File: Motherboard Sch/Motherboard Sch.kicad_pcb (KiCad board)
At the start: 2 copper layers, 117.5 x 103.5 mm, 74 parts, among them J1 DIN-5, J2 Master ISCP, J3 E SLAVE ISCP, J4 E Slave Out, J6 Pluck ISCP, J7 Pick Unit, J8 Pluck Out, J9 Power In, SW2 Master Reset, SW3 E-slave Reset, SW4 Pluck Reset, U1 PIC16F1788, U2 PIC16F1789, U3 PIC16F1789, U4 LM1117MP-1.8

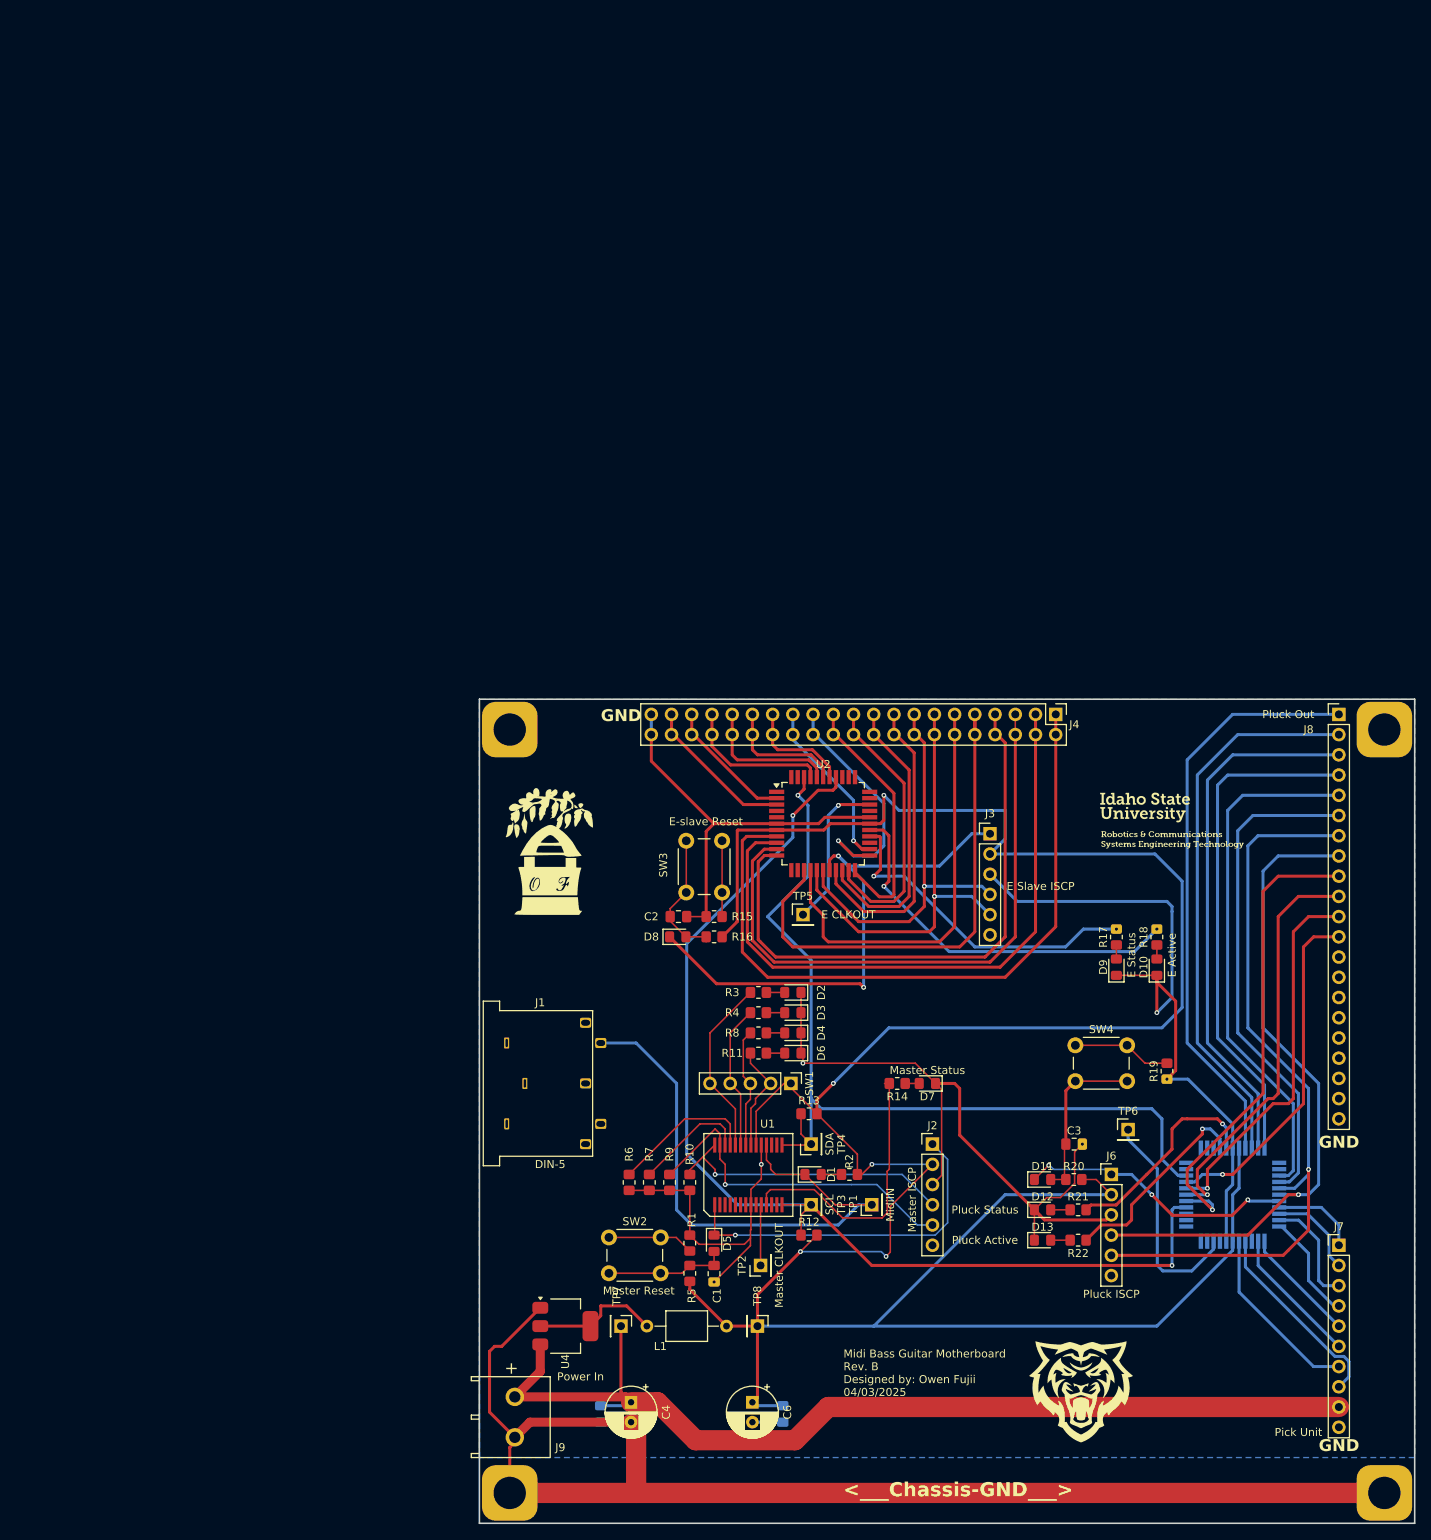
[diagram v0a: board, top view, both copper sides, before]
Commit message: added new report to repo
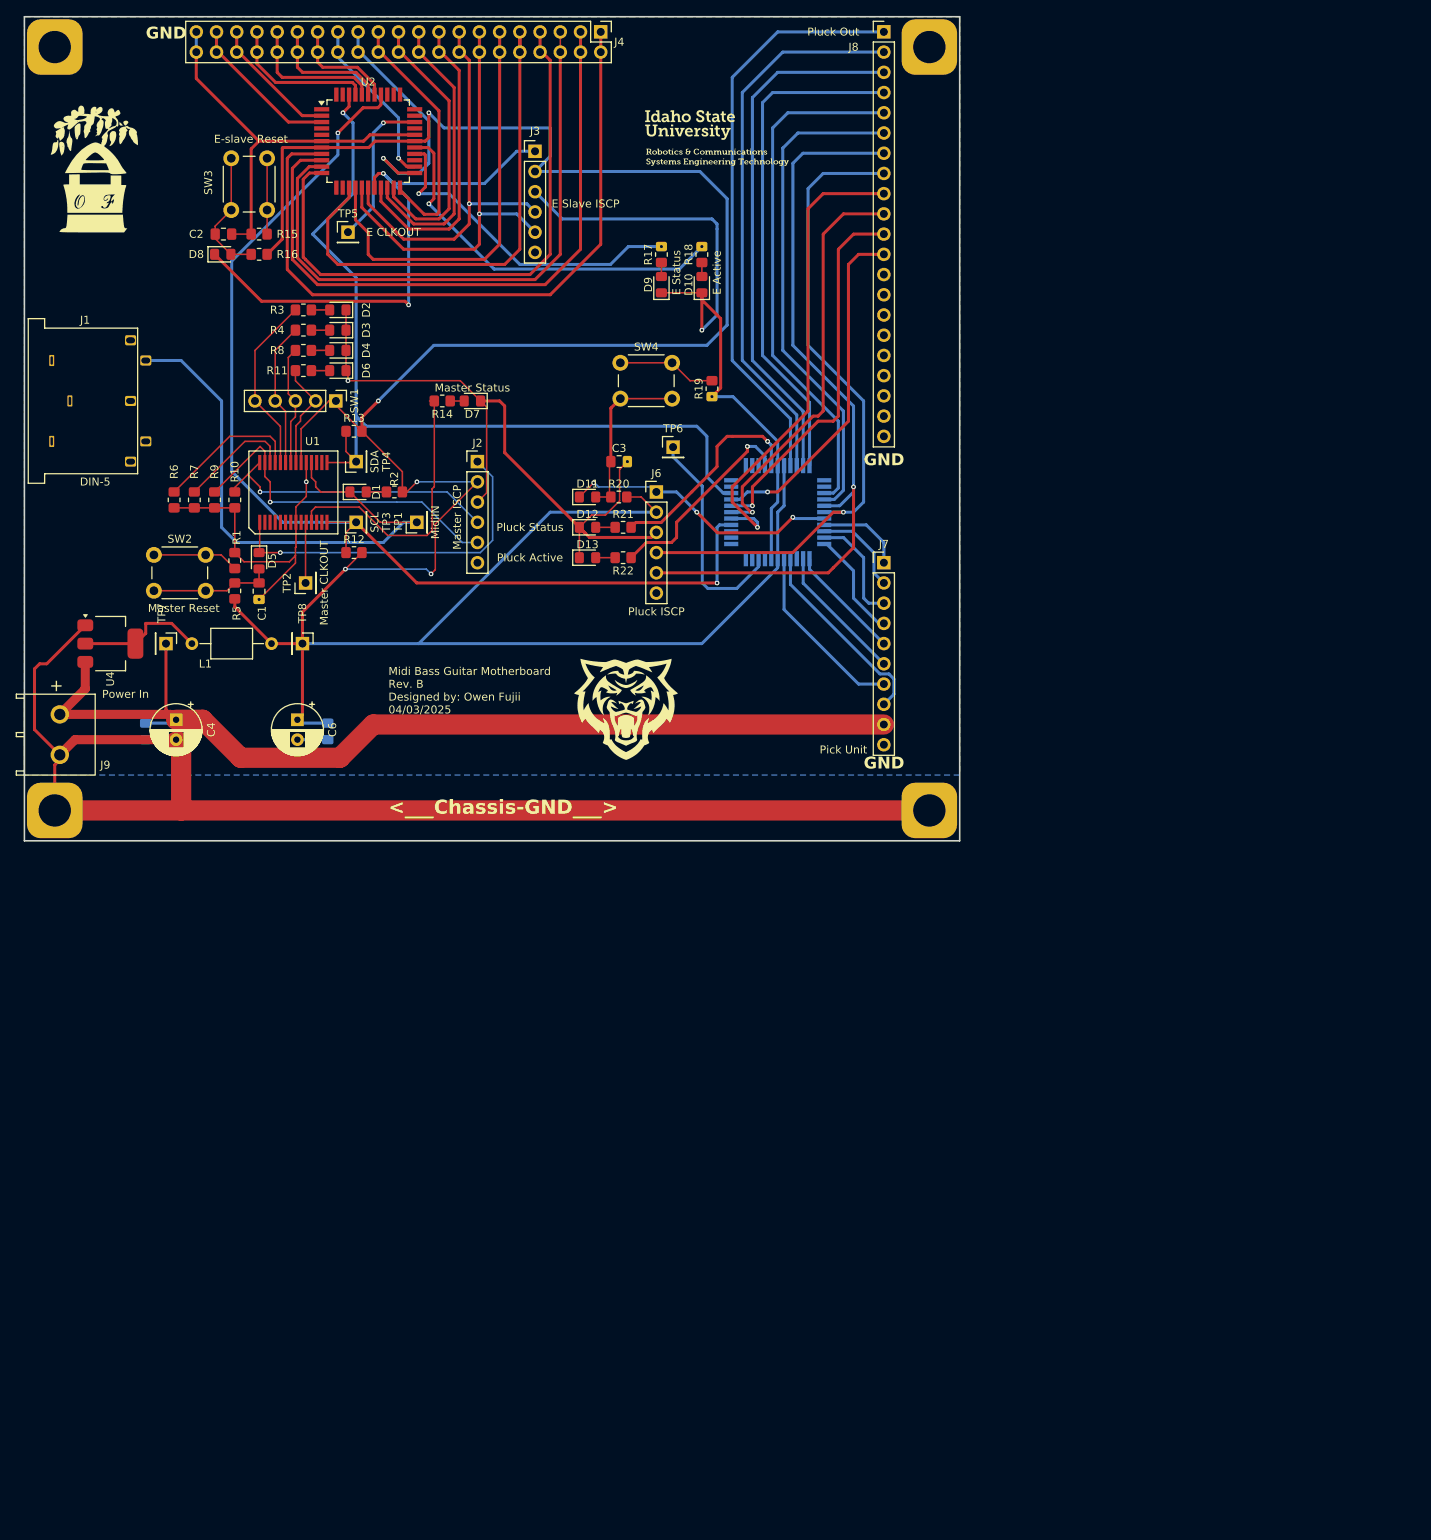
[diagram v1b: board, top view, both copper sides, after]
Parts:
- moved D11 103.0 mm to (99.3, 102.2)
- moved D12 103.0 mm to (99.3, 106.0)
- moved D13 103.0 mm to (99.3, 109.9)
- moved D2 103.0 mm to (67.9, 78.7)
- moved D6 103.0 mm to (67.9, 86.4)
- moved D7 103.0 mm to (84.8, 90.2)
- moved D9 103.0 mm to (108.6, 75.6)
- moved J1 103.0 mm to (41.9, 90.2)
- moved J3 103.0 mm to (92.7, 58.8)
- moved J7 103.0 mm to (136.5, 110.5)
- moved R11 103.0 mm to (63.6, 86.4)
- moved R13 103.0 mm to (70.0, 94.0)
- moved R14 103.0 mm to (81.1, 90.2)
- moved R17 103.0 mm to (108.6, 71.8)
- moved R21 103.0 mm to (103.8, 106.0)
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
